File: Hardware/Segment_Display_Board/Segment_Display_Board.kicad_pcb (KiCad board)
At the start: 2 copper layers, 58.4 x 141 mm, 94 parts, among them J101 IN, J102 OUT, J201 Tag Connect, J202 EXT BTN, J301 USB_B_Micro, J302 PROG, J401 19V Input, Q1001 MMBT3904, Q1002 MMBT3906, Q1101 MMBT3904, Q1102 MMBT3906, Q1201 MMBT3904, Q1202 MMBT3906, Q601 MMBT3904, Q602 MMBT3906, Q701 MMBT3904, Q702 MMBT3906, Q801 MMBT3904, Q802 MMBT3906, Q901 MMBT3904, Q902 MMBT3906, SW201 RESET, SW202 DAY_RESET, SW203 DAY_ADV, SW204 DAY_SUB, U201 ATmega328P-A, U202 DS1307Z+, U301 FT232RL, U401 NCV1117ST50T3G, U501 5inSegment, U502 SN74HC595, Y201 16mHz, Y202 32.768kHz

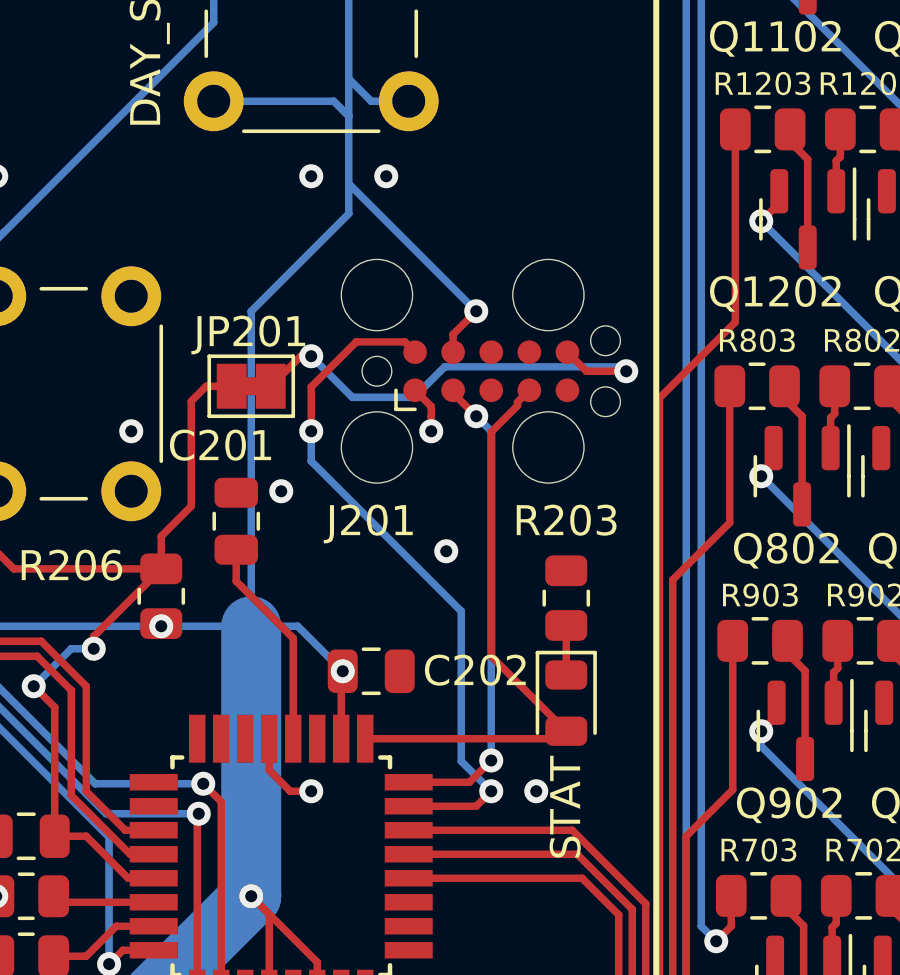
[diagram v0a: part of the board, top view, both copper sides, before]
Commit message: Possible rewire
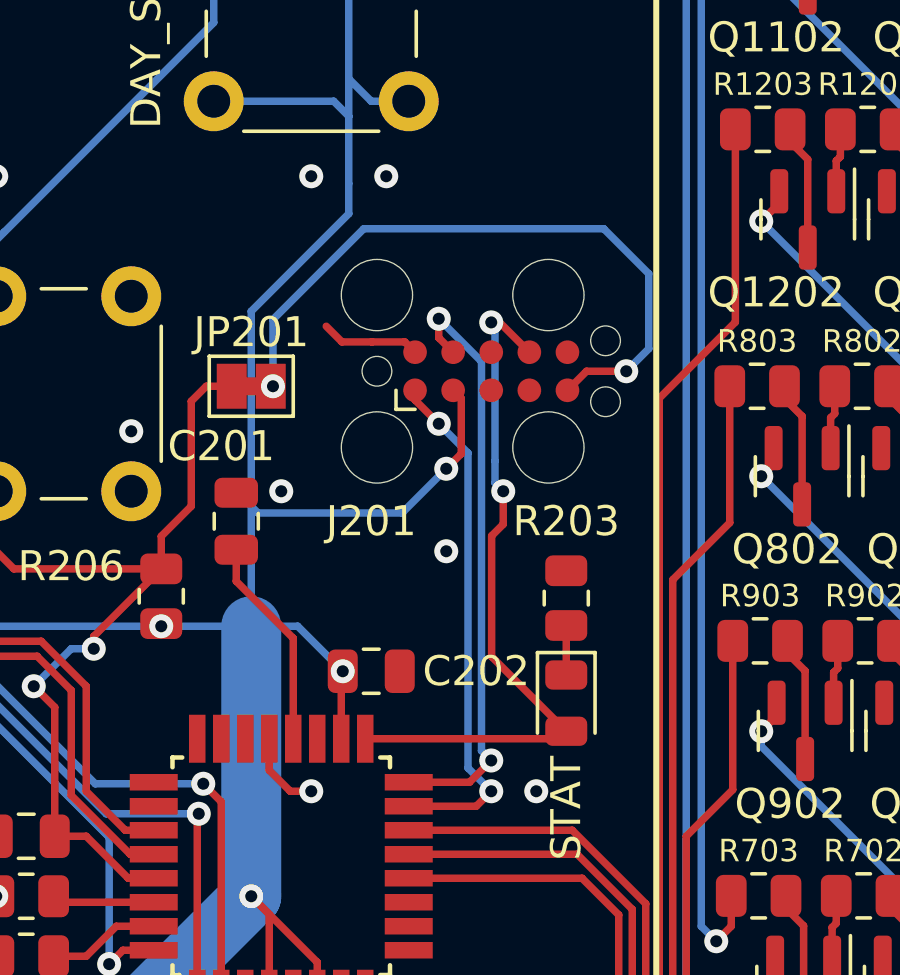
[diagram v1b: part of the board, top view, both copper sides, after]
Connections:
- J201 pad 1: GND -> /MCU/ICSP_MOSI
- J201 pad 10: /MCU/ICSP_MOSI -> GND
- J201 pad 2: /MCU/ICSP_MISO -> +5V
- J201 pad 4: /MCU/ICSP_SCK -> unconnected-(J201-Pad4)
- J201 pad 5: unconnected-(J201-Pad5) -> /MCU/ICSP_RST
- J201 pad 6: /MCU/ICSP_RST -> unconnected-(J201-Pad6)
- J201 pad 7: unconnected-(J201-Pad7) -> /MCU/ICSP_SCK
- J201 pad 9: +5V -> /MCU/ICSP_MISO
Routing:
- net /MCU/ICSP_RST: track 15.5 -> 22.5 mm
- net /MCU/ICSP_MOSI: track 23.1 -> 17.4 mm
- net /MCU/ICSP_MISO: track 15.9 -> 19.8 mm
- net /MCU/ICSP_SCK: track 19.7 -> 23.5 mm, vias 0 -> 2
- net +5V: track 315.6 -> 318.1 mm
- net GND: track 24.6 -> 26.3 mm, vias 33 -> 32
